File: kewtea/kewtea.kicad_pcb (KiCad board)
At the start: 2 copper layers, 192 x 85 mm, 62 parts, among them J1 OLED_128x32, U1 Nice_Nano_V2

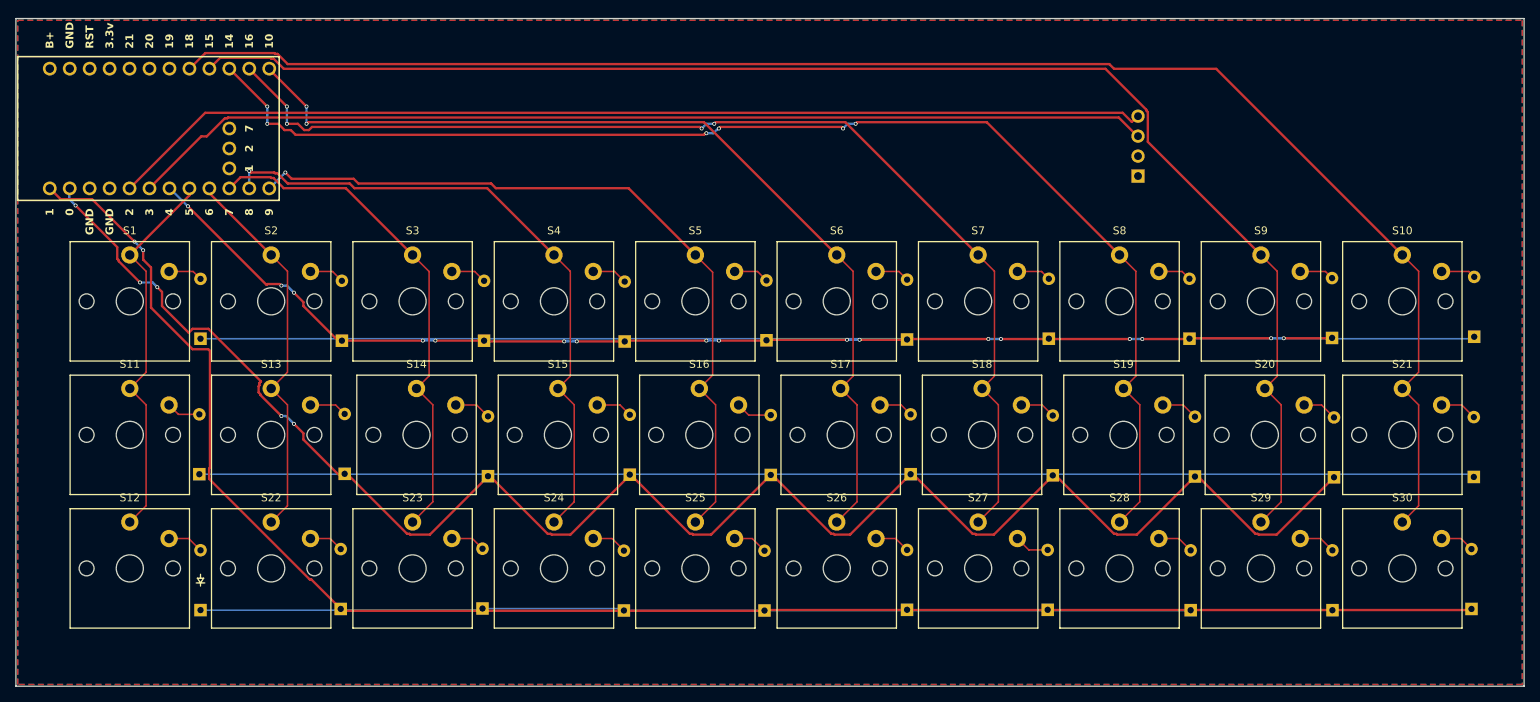
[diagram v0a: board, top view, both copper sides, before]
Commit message: add generated drill files for pcb
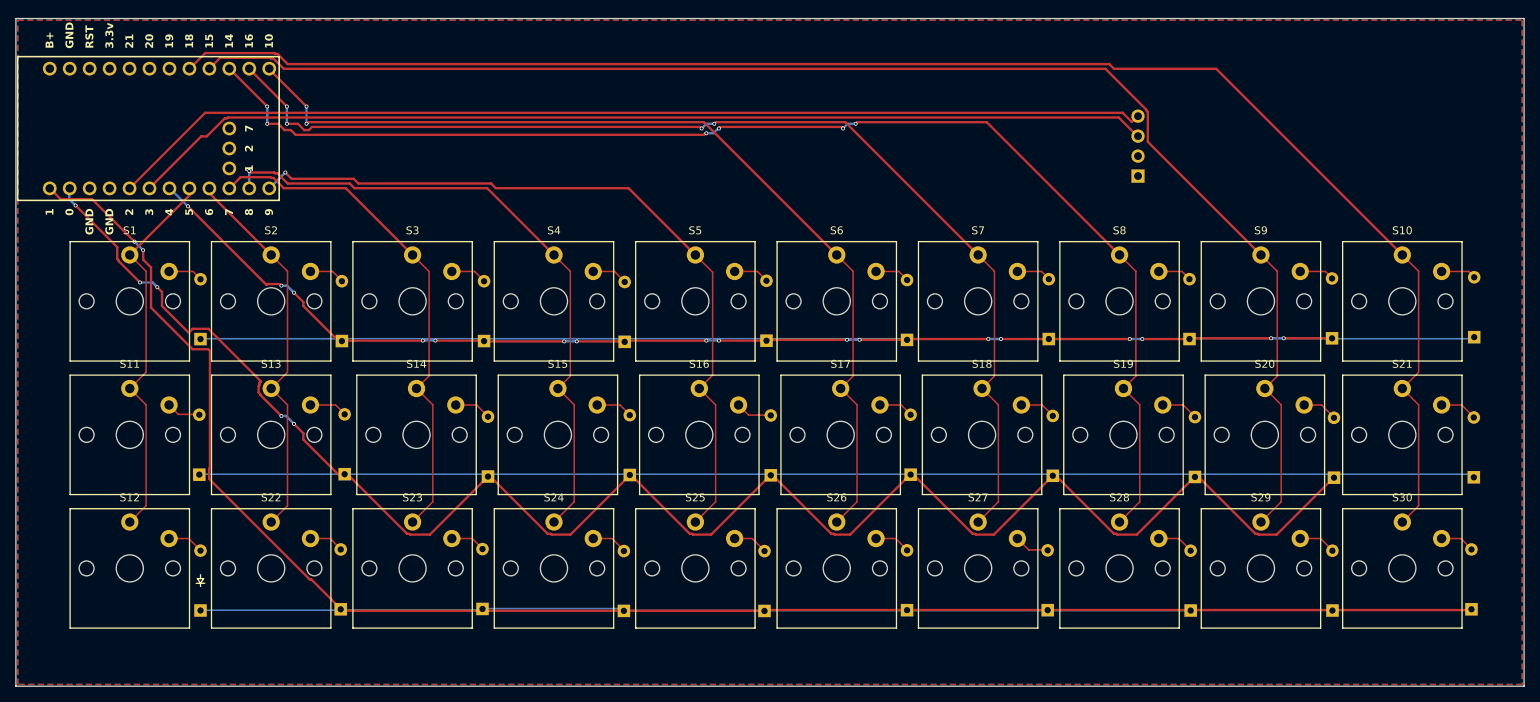
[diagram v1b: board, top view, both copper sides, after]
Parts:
- moved D13 0.05 mm to (93.8, 73.0)
- moved D16 0.05 mm to (148.1, 73.2)
- moved D28 0.05 mm to (201.6, 90.4)
- moved D29 0.05 mm to (219.6, 90.4)
- moved D1 0.05 mm to (75.5, 55.8)
- moved D10 0.05 mm to (237.7, 55.6)
- moved D2 0.05 mm to (93.5, 56.1)
- moved D3 0.05 mm to (111.6, 56.1)
- moved D9 0.05 mm to (219.6, 55.7)
